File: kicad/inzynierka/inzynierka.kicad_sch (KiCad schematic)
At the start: 17 parts

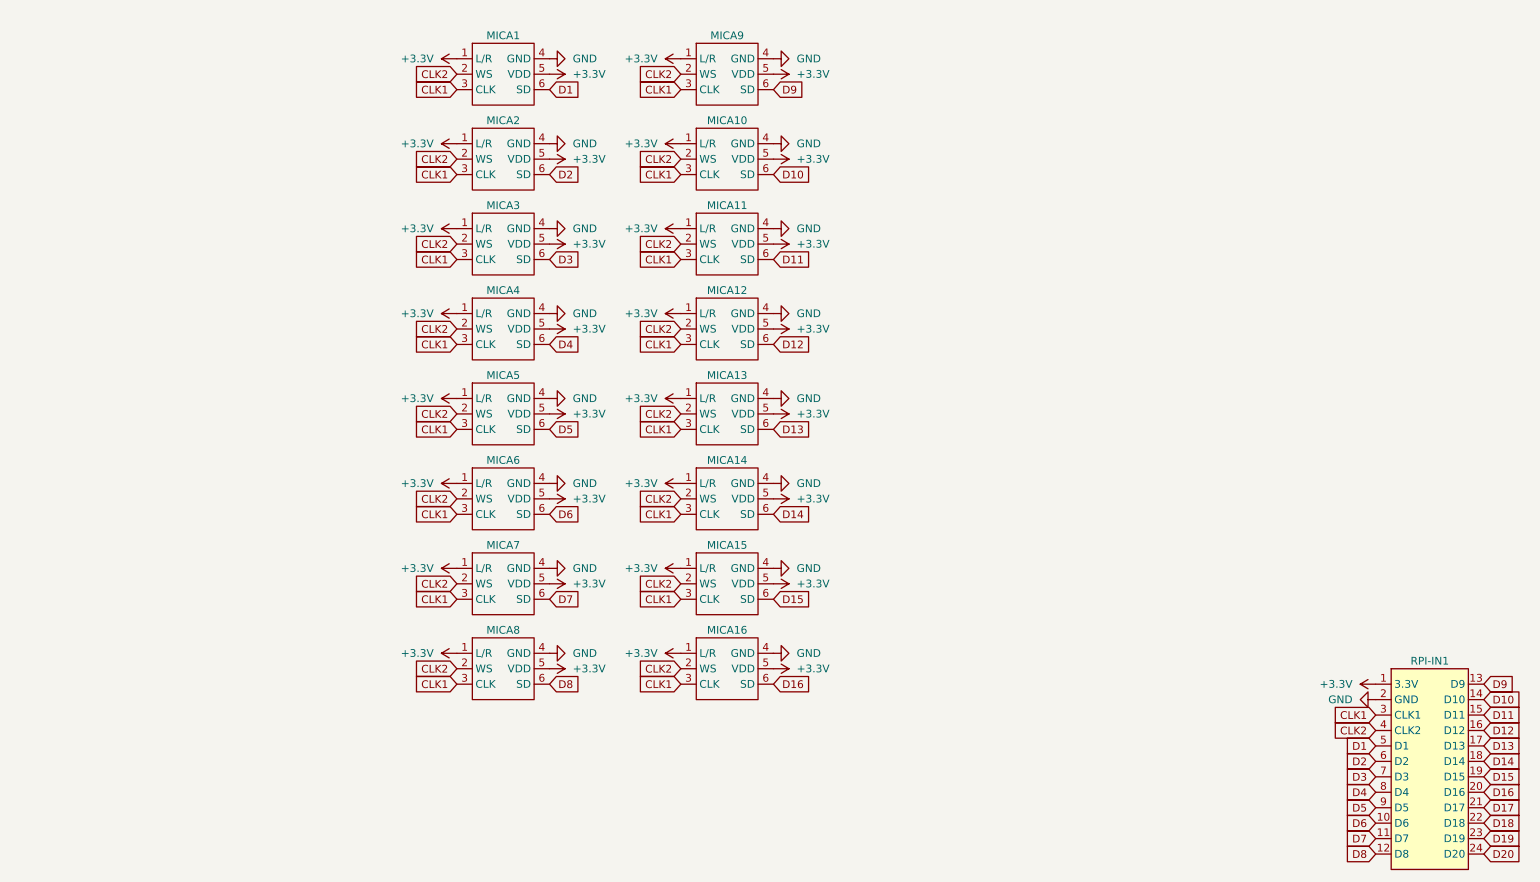
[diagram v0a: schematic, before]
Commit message: Dodanie pozycji mikrofonów B
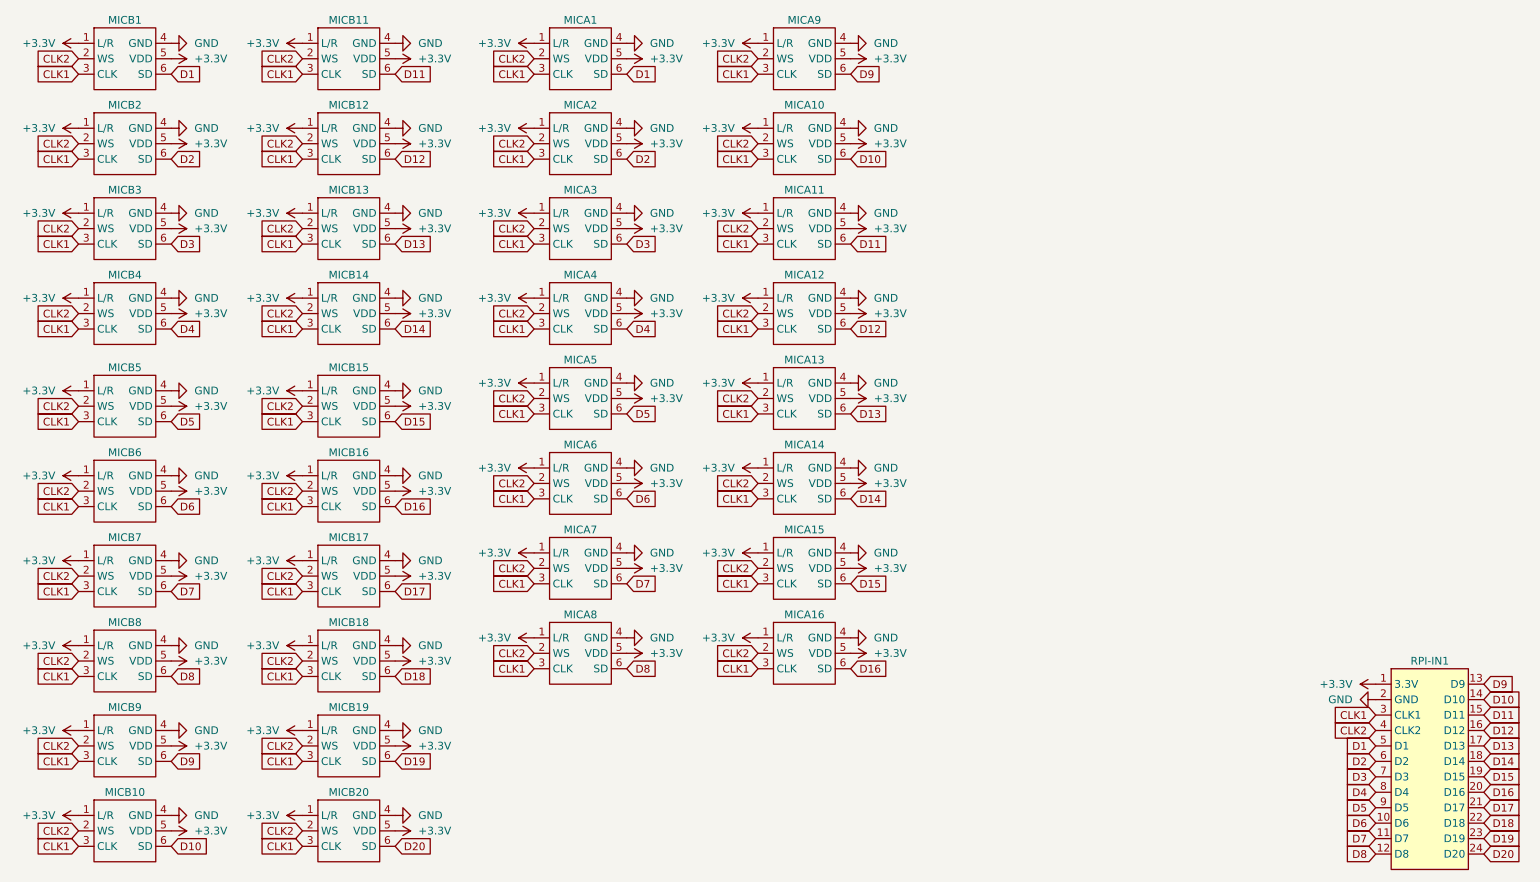
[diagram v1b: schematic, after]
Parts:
- added MICB1, MICB10, MICB11, MICB12, MICB13, MICB14, MICB15, MICB16, MICB17, MICB18, MICB19, MICB2, MICB20, MICB3, MICB4, MICB5, MICB6, MICB7, MICB8, MICB9: ~, _moje:INMP441 breakout, symbol _Moje:INMP441
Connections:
- net +3.3V: now also MICB1.1 (L/R), MICB1.5 (VDD), MICB10.1 (L/R), MICB10.5 (VDD), MICB11.1 (L/R), MICB11.5 (VDD), MICB12.1 (L/R), MICB12.5 (VDD), MICB13.1 (L/R), MICB13.5 (VDD), MICB14.1 (L/R), MICB14.5 (VDD), MICB15.1 (L/R), MICB15.5 (VDD), MICB16.1 (L/R), MICB16.5 (VDD), MICB17.1 (L/R), MICB17.5 (VDD), MICB18.1 (L/R), MICB18.5 (VDD), MICB19.1 (L/R), MICB19.5 (VDD), MICB2.1 (L/R), MICB2.5 (VDD), MICB20.1 (L/R), MICB20.5 (VDD), MICB3.1 (L/R), MICB3.5 (VDD), MICB4.1 (L/R), MICB4.5 (VDD), MICB5.1 (L/R), MICB5.5 (VDD), MICB6.1 (L/R), MICB6.5 (VDD), MICB7.1 (L/R), MICB7.5 (VDD), MICB8.1 (L/R), MICB8.5 (VDD), MICB9.1 (L/R), MICB9.5 (VDD)
- net CLK1: now also MICB1.3 (CLK), MICB10.3 (CLK), MICB11.3 (CLK), MICB12.3 (CLK), MICB13.3 (CLK), MICB14.3 (CLK), MICB15.3 (CLK), MICB16.3 (CLK), MICB17.3 (CLK), MICB18.3 (CLK), MICB19.3 (CLK), MICB2.3 (CLK), MICB20.3 (CLK), MICB3.3 (CLK), MICB4.3 (CLK), MICB5.3 (CLK), MICB6.3 (CLK), MICB7.3 (CLK), MICB8.3 (CLK), MICB9.3 (CLK)
- net CLK2: now also MICB1.2 (WS), MICB10.2 (WS), MICB11.2 (WS), MICB12.2 (WS), MICB13.2 (WS), MICB14.2 (WS), MICB15.2 (WS), MICB16.2 (WS), MICB17.2 (WS), MICB18.2 (WS), MICB19.2 (WS), MICB2.2 (WS), MICB20.2 (WS), MICB3.2 (WS), MICB4.2 (WS), MICB5.2 (WS), MICB6.2 (WS), MICB7.2 (WS), MICB8.2 (WS), MICB9.2 (WS)
- net D1: now also MICB1.6 (SD)
- net D10: now also MICB10.6 (SD)
- net D11: now also MICB11.6 (SD)
- net D12: now also MICB12.6 (SD)
- net D13: now also MICB13.6 (SD)
- net D14: now also MICB14.6 (SD)
- net D15: now also MICB15.6 (SD)
- net D16: now also MICB16.6 (SD)
- net D17: now also MICB17.6 (SD)
- net D18: now also MICB18.6 (SD)
- net D19: now also MICB19.6 (SD)
- net D2: now also MICB2.6 (SD)
- net D20: now also MICB20.6 (SD)
- net D3: now also MICB3.6 (SD)
- net D4: now also MICB4.6 (SD)
- net D5: now also MICB5.6 (SD)
- net D6: now also MICB6.6 (SD)
- net D7: now also MICB7.6 (SD)
- net D8: now also MICB8.6 (SD)
- net D9: now also MICB9.6 (SD)
- net GND: now also MICB1.4 (GND), MICB10.4 (GND), MICB11.4 (GND), MICB12.4 (GND), MICB13.4 (GND), MICB14.4 (GND), MICB15.4 (GND), MICB16.4 (GND), MICB17.4 (GND), MICB18.4 (GND), MICB19.4 (GND), MICB2.4 (GND), MICB20.4 (GND), MICB3.4 (GND), MICB4.4 (GND), MICB5.4 (GND), MICB6.4 (GND), MICB7.4 (GND), MICB8.4 (GND), MICB9.4 (GND)
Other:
- moved on the sheet: MICA1, MICA10, MICA11, MICA12, MICA13, MICA14, MICA15, MICA16, MICA2, MICA3, MICA4, MICA5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
